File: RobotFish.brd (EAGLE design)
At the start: 160 x 100 mm, 36 parts, among them U1 16F1575, U2 MCP73831/OT, U3 MCP1754S_SOT23, X1 JST_3PIN

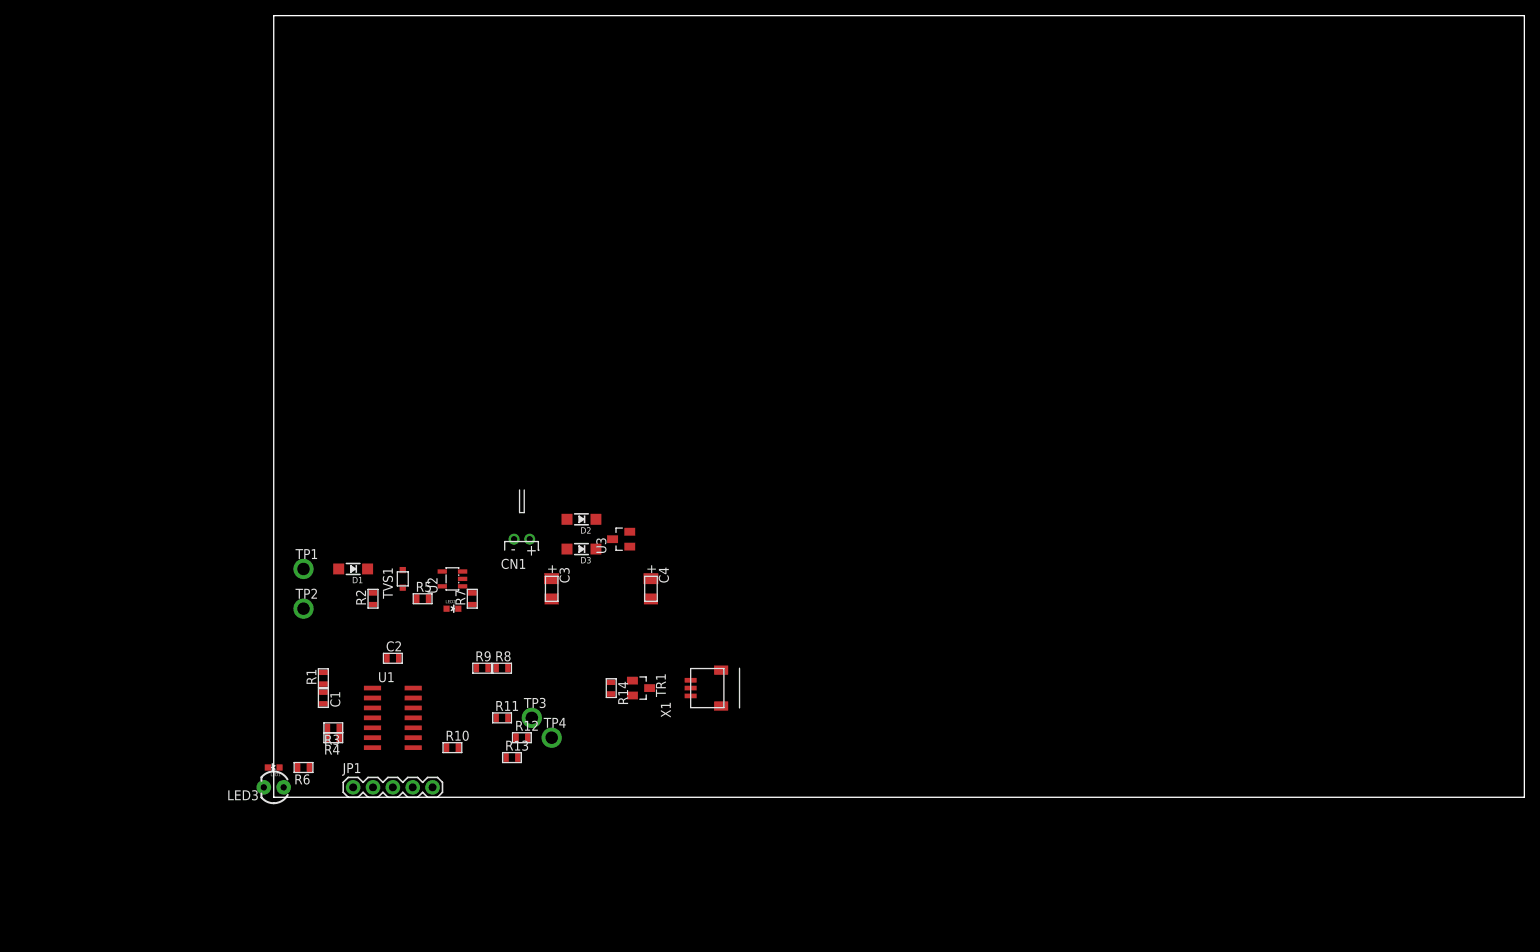
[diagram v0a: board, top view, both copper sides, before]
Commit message: gerber done
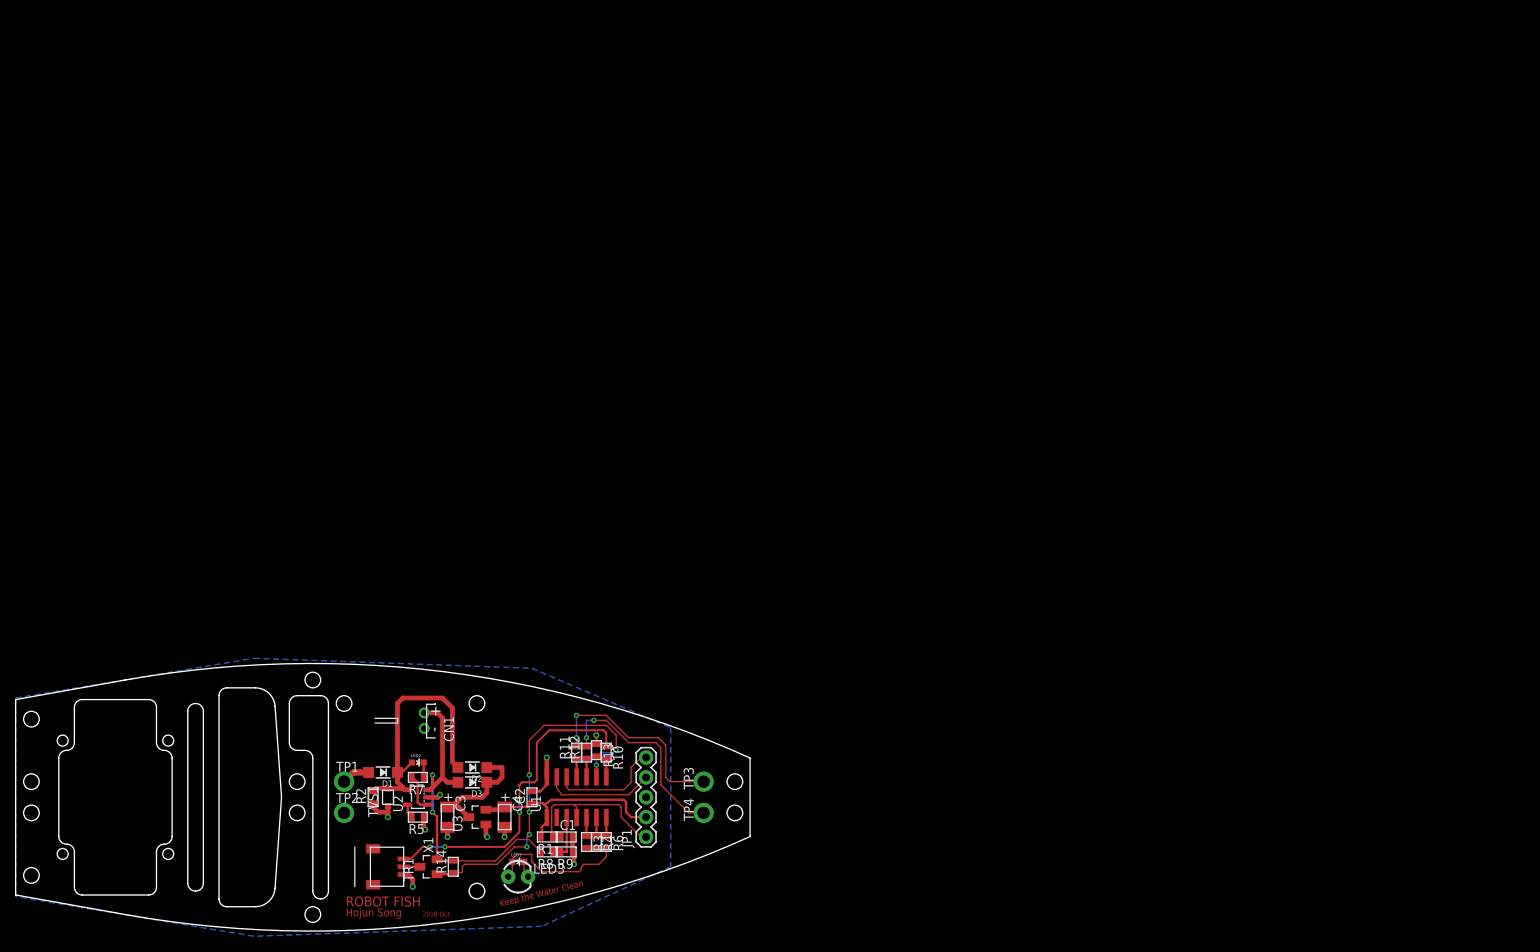
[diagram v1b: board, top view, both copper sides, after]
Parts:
- moved X1 43.3 mm to (16.6, -8.89), turned to 270 degrees
- moved U3 40.0 mm to (26.1, -2.54)
- moved R6 39.9 mm to (42.6, -5.71), turned to 270 degrees
- moved JP1 38.0 mm to (47.6, -5.08), turned to 90 degrees
- moved R4 36.2 mm to (41.3, -5.71), turned to 270 degrees
- moved C1 35.8 mm to (37.5, -5.08), turned to 0 degrees
- moved R3 35.5 mm to (40.0, -5.71), turned to 270 degrees
- moved TR1 35.5 mm to (19.8, -8.89), turned to 90 degrees
- moved R1 35.1 mm to (34.9, -5.08), turned to 180 degrees
- moved C4 34.7 mm to (29.5, -2.54)
- moved D2 34.7 mm to (25.4, 3.81)
- moved LED1 33.5 mm to (31.3, -8.26), turned to 270 degrees
- moved LED3 33.3 mm to (31.3, -10.2), turned to 0 degrees
- moved D3 32.9 mm to (25.4, 1.91)
- moved C3 32.1 mm to (22.2, -2.54)
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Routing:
- net SERVO_ON: track 0.00 -> 46.8 mm, vias 0 -> 6
- net VBAT: track 0.00 -> 42.8 mm, vias 0 -> 2
- net SERVO_PWM: track 0.00 -> 41.0 mm, vias 0 -> 4
- net +5V: track 0.00 -> 33.9 mm
- net +3.3V: track 0.00 -> 27.5 mm
- net DGND: track 0.00 -> 26.7 mm, vias 0 -> 10
- net N$15: track 0.00 -> 26.2 mm, vias 0 -> 2
- net N$16: track 0.00 -> 26.1 mm, vias 0 -> 2
- net RESET: track 0.00 -> 21.4 mm
- net N$8: track 0.00 -> 18.5 mm
- net VIN: track 0.00 -> 15.1 mm
- net ICSPCLK: track 0.00 -> 14.5 mm
- net ICSPDAT: track 0.00 -> 14.2 mm
- net BAT_ADC: track 0.00 -> 6.17 mm
- net N$2: track 0.00 -> 4.98 mm
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- added copper zone on layer 16, net DGND
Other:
- board size 160 x 100 mm -> 94 x 34.2 mm
- board text added: "2016 Oct"
- board text added: "Hojun Song"
- board text added: "Keep the Water Clean"
- board text added: "ROBOT FISH"

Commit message: value changed
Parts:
- R10, R3, R4: value (none) -> 4.7k
- R2: value 100k -> 1M
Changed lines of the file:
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@@
 <element name="D2" library="microbuilder" package="SOD-123" value="MBR120" x="25.415" y="3.81" rot="R180"/>
 <element name="U1" library="water" package="SO-14" value="16F1575" x="38.75" y="0"/>
-<element name="R2" library="water" package="R0603(1608)" value="100k" x="12.715" y="0" rot="R90"/>
+<element name="R2" library="water" package="R0603(1608)" value="1M" x="12.715" y="0" rot="R90"/>
 <element name="TR1" library="water" package="SOT23" value="SSM3J338R" x="19.795" y="-8.89" rot="R90"/>
 <element name="R14" library="water" package="R0603(1608)" value="100k" x="22.97" y="-8.89" rot="R90"/>
 <element name="C2" library="water" package="C0603(1608)" value="0.1uF" x="33.035" y="0" rot="R90"/>
-<element name="R10" library="water" package="R0603(1608)" value="" x="42.53" y="5.715" rot="R270"/>
+<element name="R10" library="water" package="R0603(1608)" value="4.7k" x="42.53" y="5.715" rot="R270"/>
 <element name="R1" library="water" package="R0603(1608)" value="100k" x="34.94" y="-5.08" rot="R180"/>
 <element name="C1" library="water" package="C0603(1608)" value="0.1uF" x="37.48" y="-5.08"/>
 <element name="D1" library="microbuilder" package="SOD-123" value="MBR120" x="13.985" y="3.175" rot="R180"/>
-<element name="R3" library="water" package="R0603(1608)" value="" x="40.02" y="-5.715" rot="R270"/>
-<element name="R4" library="water" package="R0603(1608)" value="" x="41.29" y="-5.715" rot="R270"/>
+<element name="R3" library="water" package="R0603(1608)" value="4.7k" x="40.02" y="-5.715" rot="R270"/>
+<element name="R4" library="water" package="R0603(1608)" value="4.7k" x="41.29" y="-5.715" rot="R270"/>
 <element name="R6" library="water" package="R0603(1608)" value="1k" x="42.56" y="-5.715" rot="R270"/>
 <element name="LED1" library="berry" package="LED-0603" value="" x="31.2725" y="-8.255" rot="R270"/>
